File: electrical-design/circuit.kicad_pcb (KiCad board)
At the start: 4 copper layers, 100 x 70 mm, 48 parts, among them J1 AVR-ISP-10, J2 Conn_01x03_Female, Q1 2N3906, Q2 2N3906, Q3 2N3906, Q4 2N3906, SW1 SW_Push, SW2 SW_DIP_x04, SW3 SW_Push, U1 ATmega8A-P, U2 LTC-4627JD, U3 NE555P, Y1 16MHz

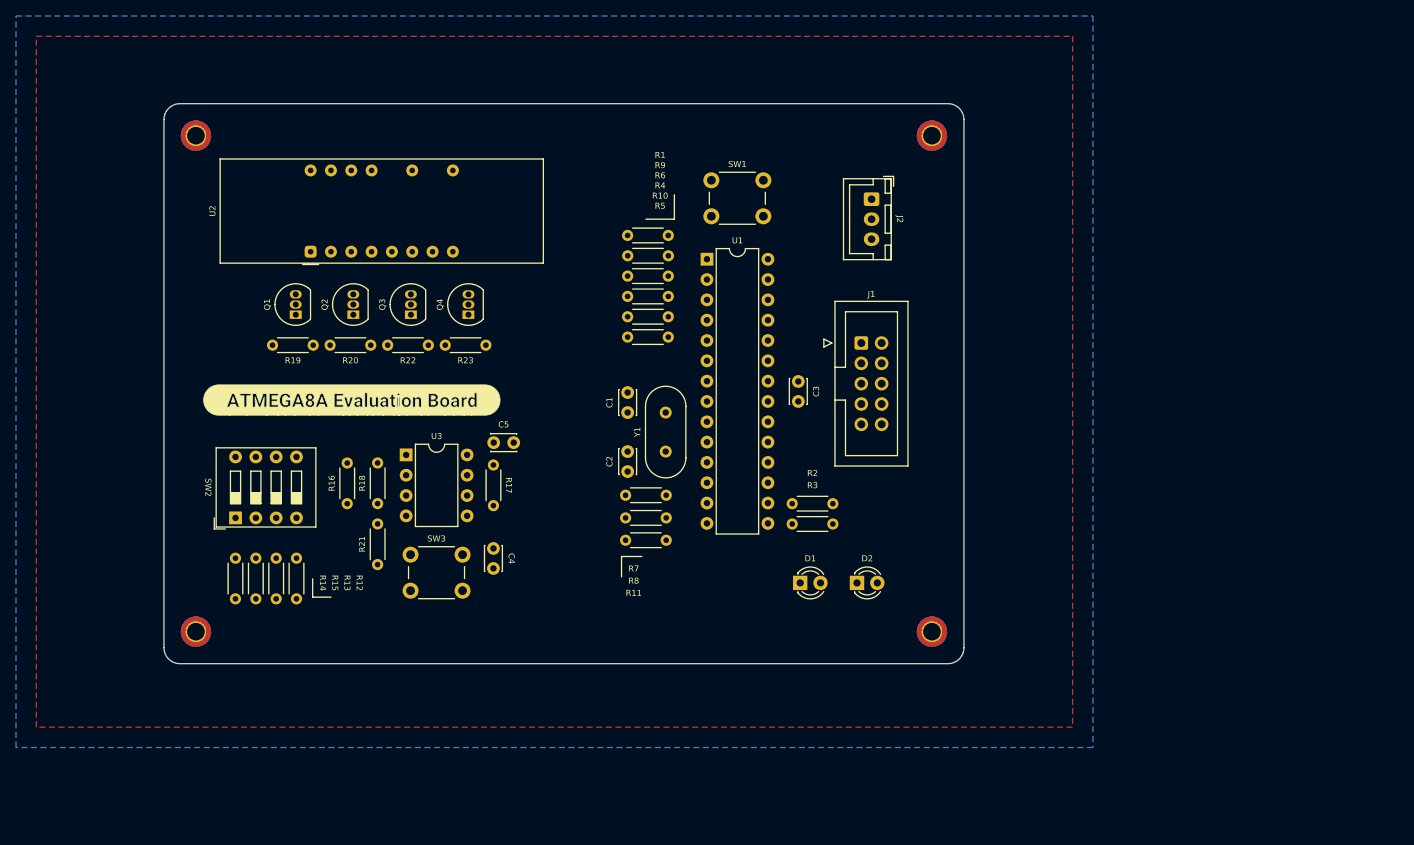
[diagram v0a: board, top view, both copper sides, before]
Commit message: Completed Initial Design of Circuit Board
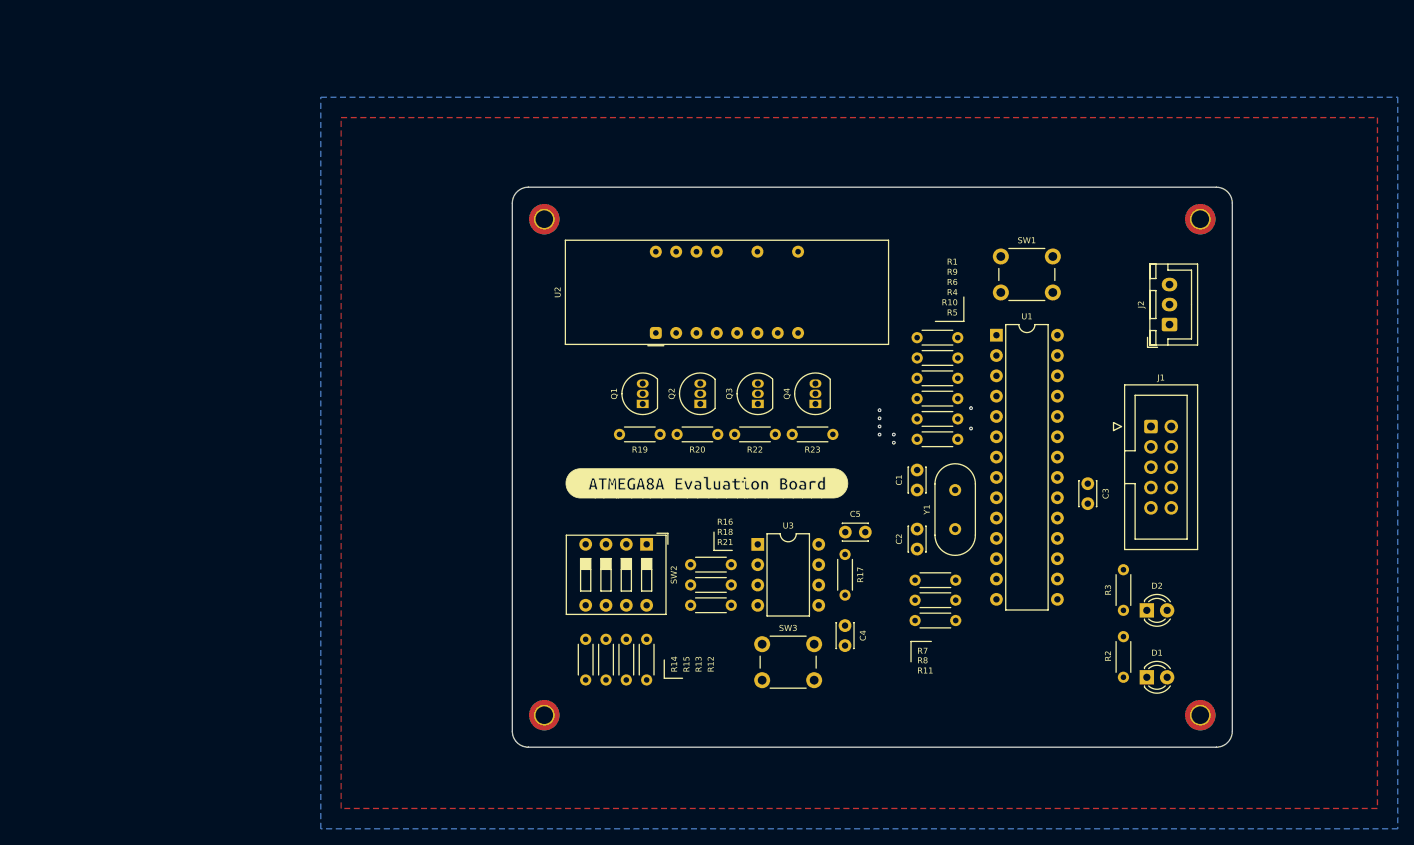
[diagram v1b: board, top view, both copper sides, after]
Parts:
- removed kibuzzard-63E126FF: G***, kibuzzard-63E126FF
- added kibuzzard-63E387B9: G***, kibuzzard-63E387B9, F.Cu at (81.3, 61.0)
- moved H4 126.0 mm to (143.0, 27.9)
- moved SW2 51.5 mm to (73.8, 68.6), turned to -90 degrees
- moved H3 49.6 mm to (61.0, 27.9)
- moved R2 46.7 mm to (133.3, 85.2), turned to 90 degrees
- moved C5 45.4 mm to (98.6, 67.1)
- moved U3 45.4 mm to (87.6, 68.6)
- moved R17 45.4 mm to (98.6, 69.8)
- moved SW3 45.4 mm to (88.2, 81.1)
- moved C4 45.0 mm to (98.6, 78.7)
- moved R15 44.9 mm to (66.1, 85.5)
- moved R12 44.9 mm to (73.8, 85.5)
- moved R14 44.9 mm to (68.7, 85.5)
- moved R13 44.9 mm to (71.2, 85.5)
- moved D1 44.9 mm to (136.3, 85.2)
- moved Q3 44.8 mm to (87.7, 51.0)
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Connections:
- net A renamed /A
- net B renamed /B
- net C renamed /C
- net D renamed /D
- net DECIMAL renamed /DEC
- net E renamed /E
- net F renamed /F
- net G renamed /G
- C3 pad 1: GND -> Net-(C3-Pad1)
- C3 pad 2: Net-(C3-Pad2) -> GND
- D1 pad 1: GND -> Net-(D1-Pad1)
- D1 pad 2: Net-(D1-Pad2) -> Net-(U1-Pad15)
- D2 pad 1: GND -> Net-(D2-Pad1)
- D2 pad 2: Net-(D2-Pad2) -> Net-(U1-Pad16)
- R12 pad 2: Net-(R12-Pad2) -> Net-(SW2-Pad8)
- R13 pad 2: Net-(R13-Pad2) -> Net-(SW2-Pad7)
- R14 pad 2: Net-(R14-Pad2) -> Net-(SW2-Pad6)
- R15 pad 2: Net-(R15-Pad2) -> Net-(SW2-Pad5)
- R18 pad 1: Frequency -> VCC
- R18 pad 2: VCC -> Frequency
- R2 pad 1: Net-(U1-Pad15) -> Net-(D1-Pad1)
- R2 pad 2: Net-(D1-Pad2) -> GND
- R3 pad 1: Net-(U1-Pad16) -> Net-(D2-Pad1)
- R3 pad 2: Net-(D2-Pad2) -> GND
- SW2 pad 1: Net-(R15-Pad2) -> Net-(R16-Pad2)
- SW2 pad 2: Net-(R14-Pad2) -> Net-(R16-Pad2)
- SW2 pad 3: Net-(R13-Pad2) -> Net-(R16-Pad2)
- SW2 pad 4: Net-(R12-Pad2) -> Net-(R16-Pad2)
- SW2 pad 5: Net-(R16-Pad2) -> Net-(SW2-Pad5)
- SW2 pad 6: Net-(R16-Pad2) -> Net-(SW2-Pad6)
- SW2 pad 7: Net-(R16-Pad2) -> Net-(SW2-Pad7)
- SW2 pad 8: Net-(R16-Pad2) -> Net-(SW2-Pad8)
- U1 pad 21: Net-(C3-Pad2) -> Net-(C3-Pad1)
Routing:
- net Net-(U1-Pad15): track 0.00 -> 17.8 mm
- net Net-(J2-Pad2): track 0.00 -> 16.7 mm
- net Net-(U1-Pad16): track 0.00 -> 15.3 mm
- net ~{DIGIT_3}: track 39.7 -> 31.1 mm, vias 0 -> 2
- net ~{RESET}: track 38.4 -> 45.2 mm
- net Net-(R4-Pad2): track 41.5 -> 35.2 mm
- net Net-(R6-Pad2): track 37.9 -> 31.6 mm
- net Net-(R9-Pad2): track 31.8 -> 25.5 mm
- net ~{DIGIT_2}: track 45.4 -> 39.6 mm, vias 0 -> 2
- net Net-(R21-Pad2): track 9.07 -> 14.9 mm
- net Net-(R15-Pad2): track 5.04 -> 0.00 mm
- net Net-(R14-Pad2): track 5.04 -> 0.00 mm
- net Net-(R13-Pad2): track 5.04 -> 0.00 mm
- net Net-(R12-Pad2): track 5.04 -> 0.00 mm
- net Net-(R10-Pad2): track 44.7 -> 40.0 mm
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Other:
- board size 100 x 70 mm -> 90 x 70 mm

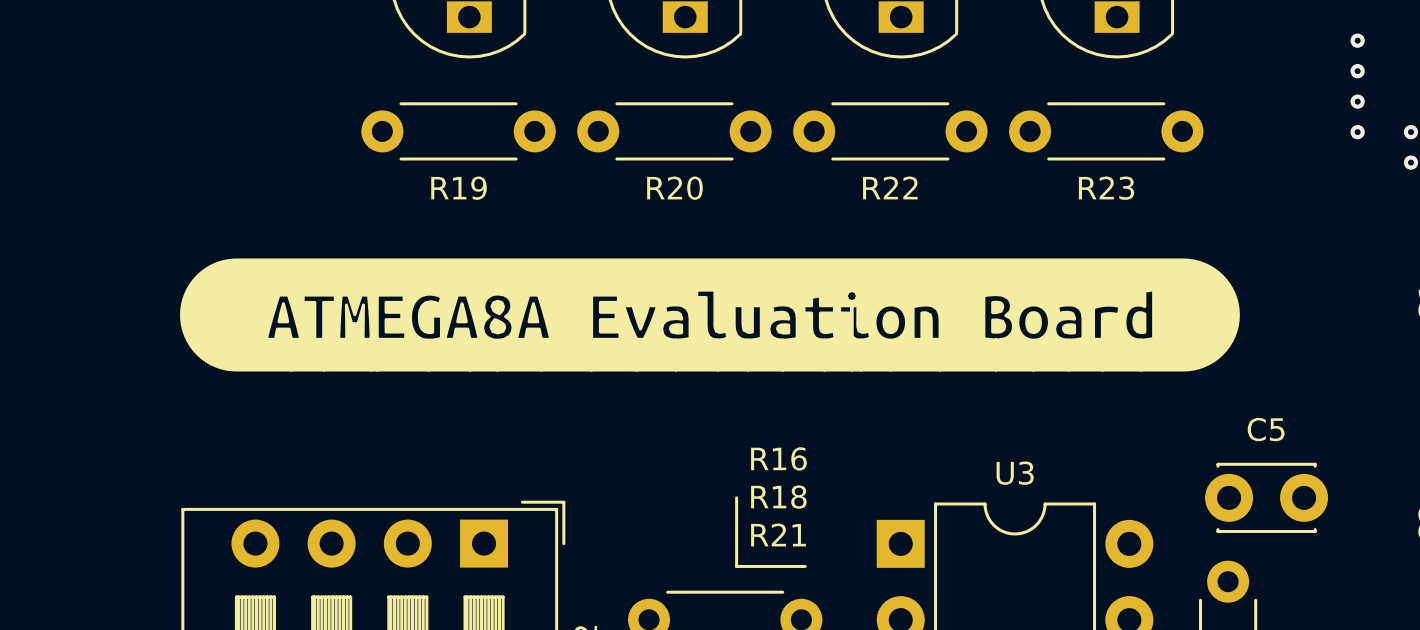
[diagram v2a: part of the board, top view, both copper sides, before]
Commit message: Commiting Missing Files
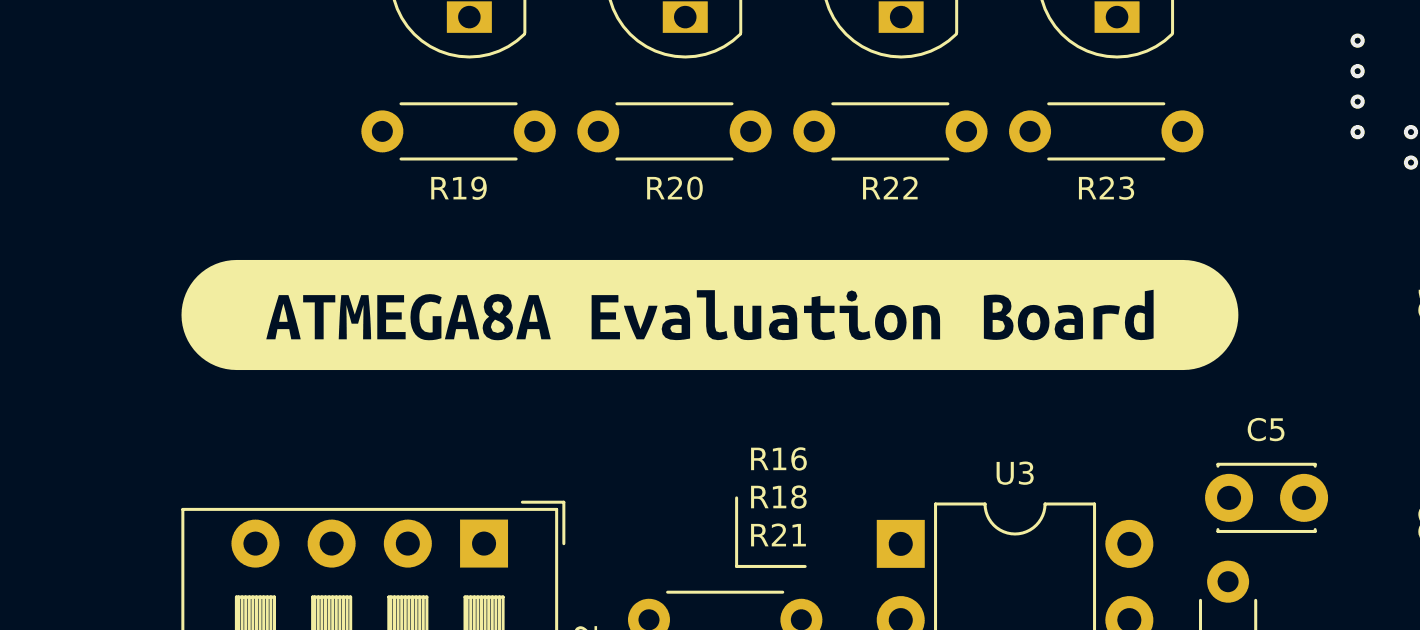
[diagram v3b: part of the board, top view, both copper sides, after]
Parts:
- removed kibuzzard-63E387B9: G***, kibuzzard-63E387B9
- added kibuzzard-63E778F7: G***, kibuzzard-63E778F7, F.Cu at (81.3, 61.0)

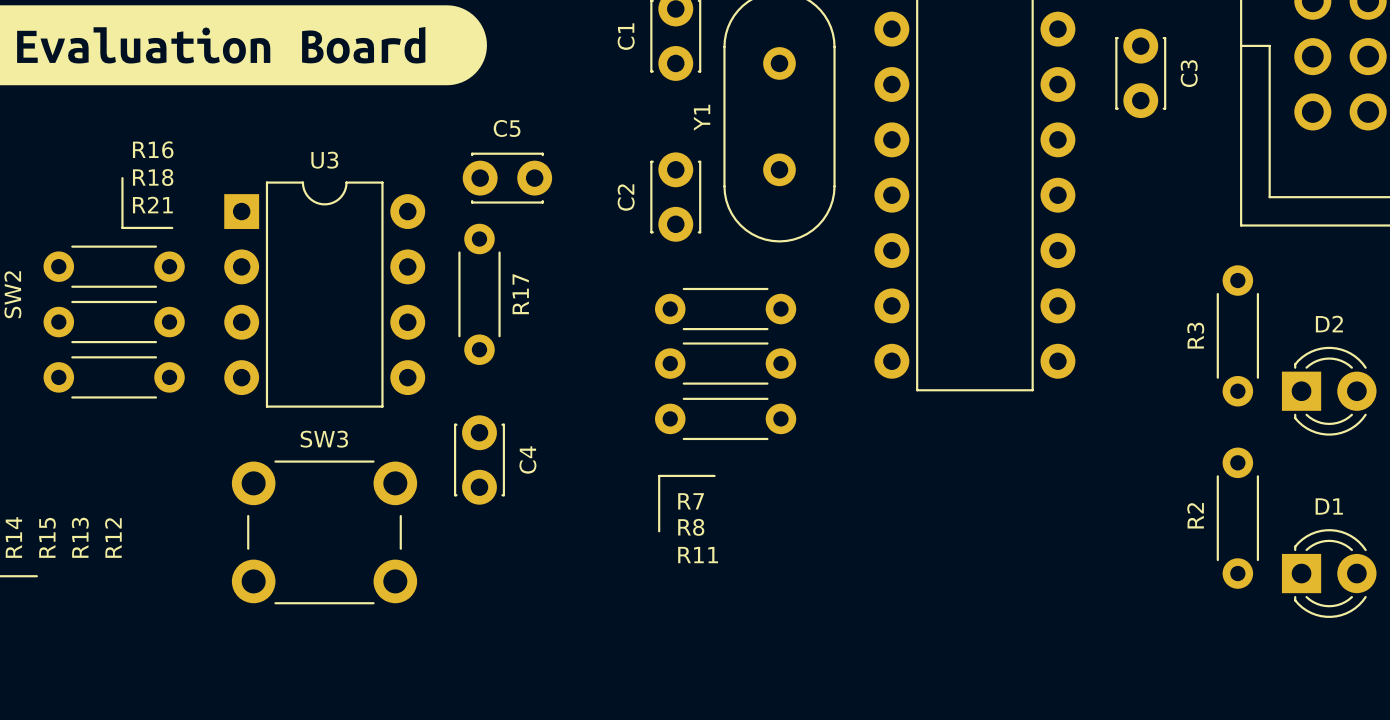
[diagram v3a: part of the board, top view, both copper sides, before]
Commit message: Added Production Files
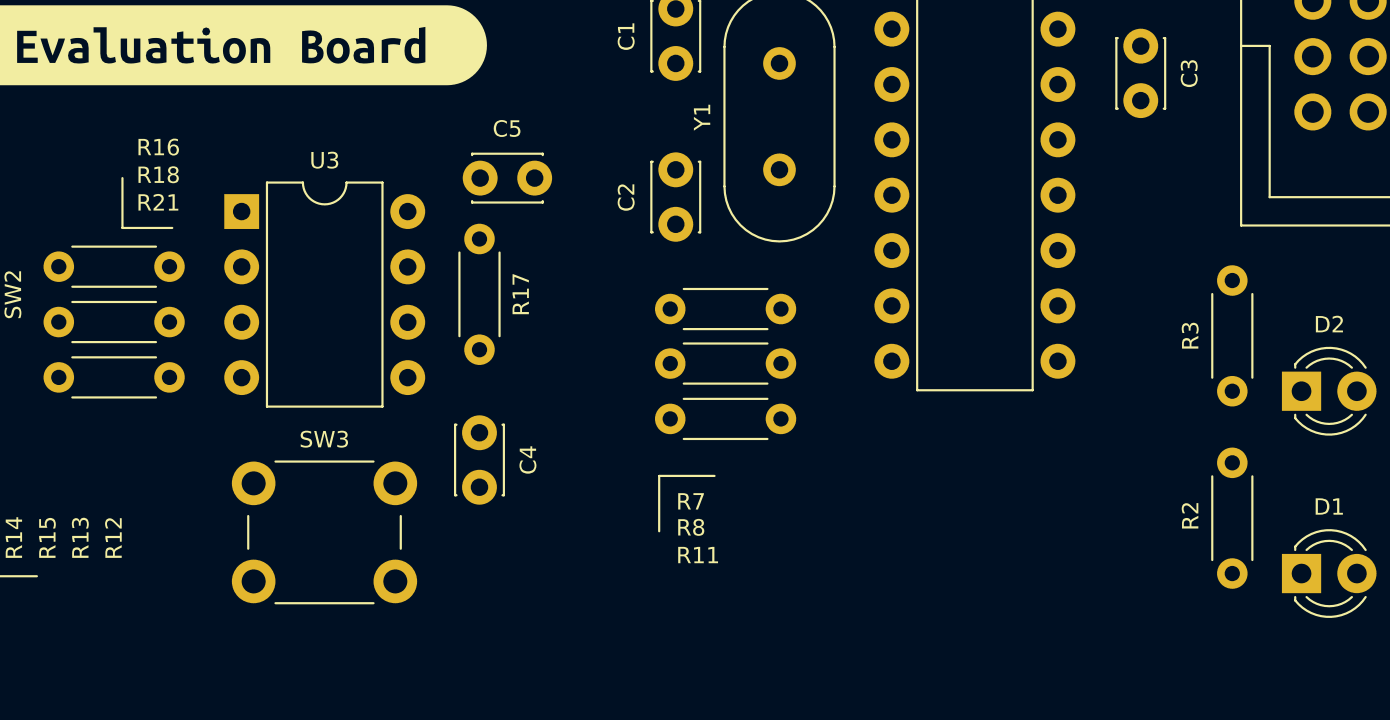
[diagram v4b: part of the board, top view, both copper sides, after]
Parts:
- moved R2 0.25 mm to (133.1, 85.2)
- moved R3 0.25 mm to (133.1, 76.8)
